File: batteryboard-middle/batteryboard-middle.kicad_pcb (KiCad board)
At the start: 2 copper layers, 46.8 x 46.8 mm, 8 parts, among them J1 Conn_02x05_Odd_Even, J2 Conn_01x02, J3 Conn_01x02, J4 Conn_02x05_Odd_Even

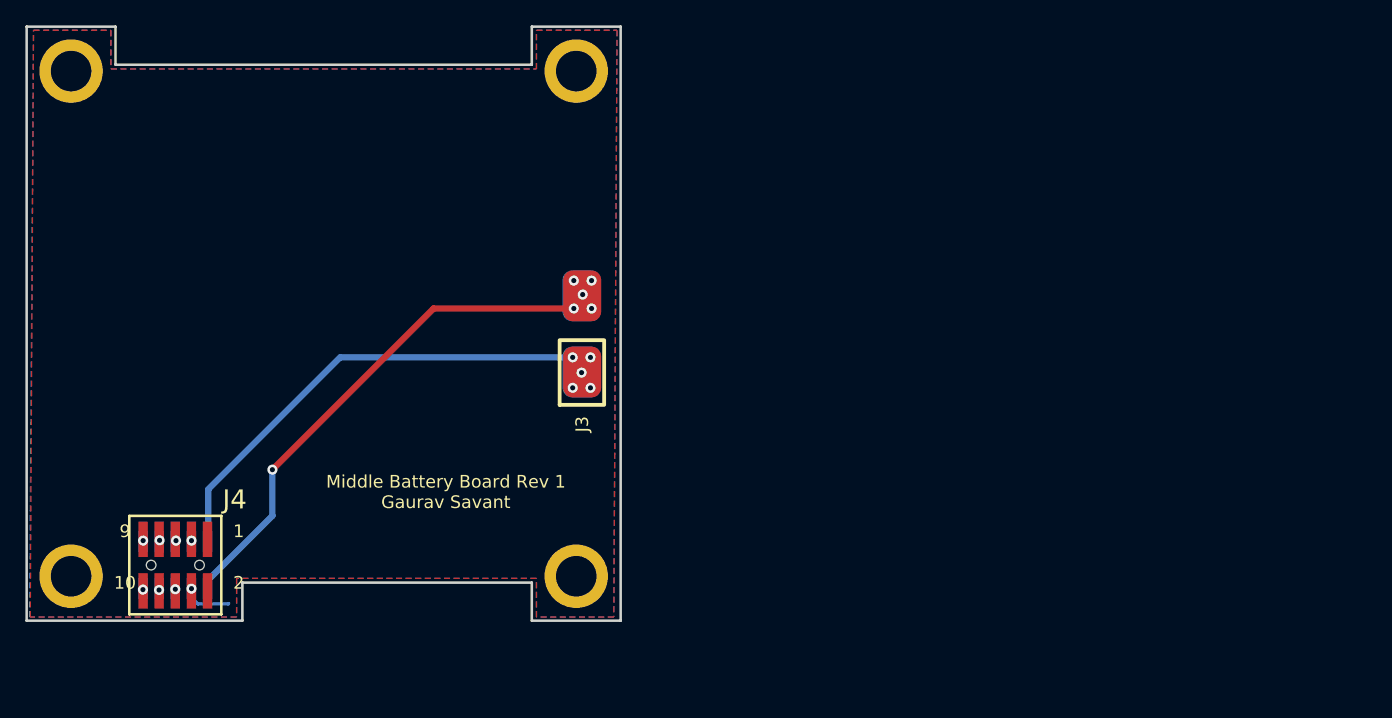
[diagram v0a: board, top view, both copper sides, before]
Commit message: Fixes and cleanup
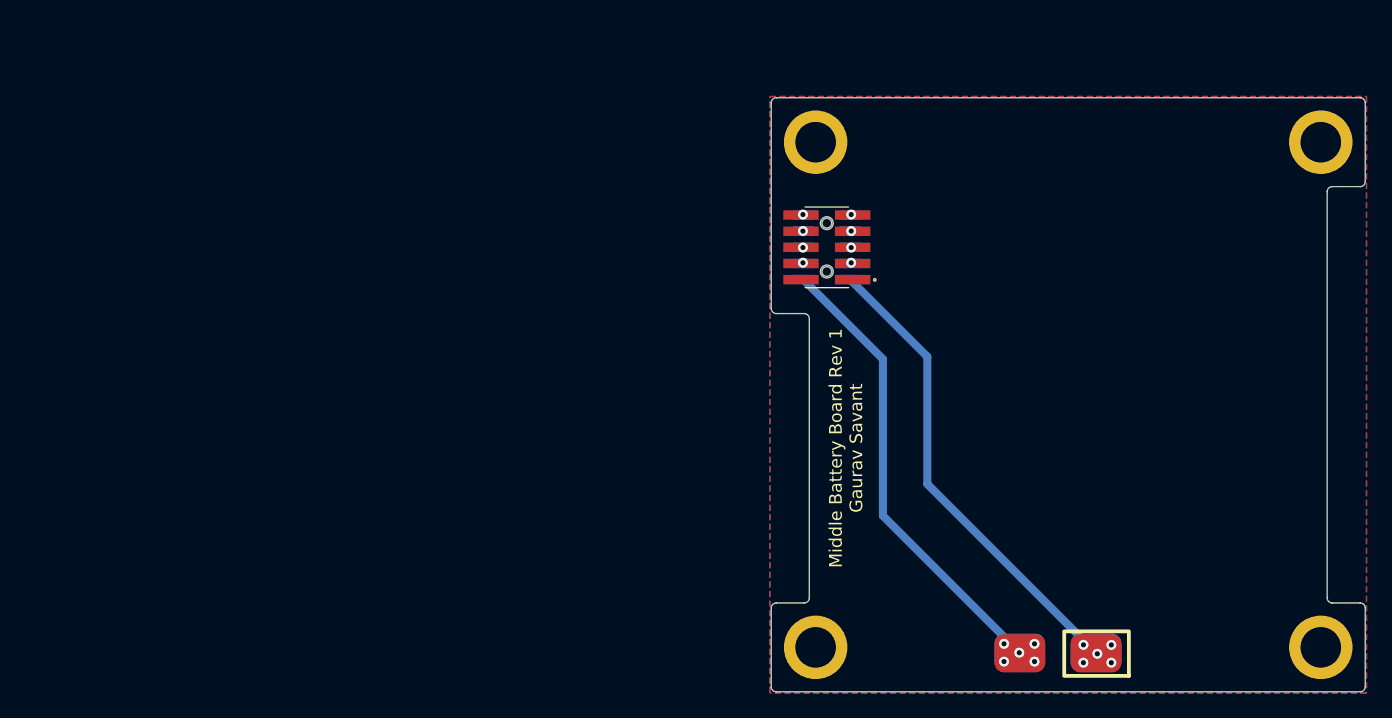
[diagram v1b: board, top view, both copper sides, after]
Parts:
- added Ref**: Val**, custom-footprints:pycubed_mini_half, F.Cu at (147.6, 80.2)
- J4: footprint batteryboard:SAMTEC-FTS-105-01-X-DV -> batteryboard:FTS-105-XX-YY-DV-A
- moved H1 98.6 mm to (166.7, 80.7), turned to -90 degrees
- moved H2 74.2 mm to (166.7, 120.5), turned to -90 degrees
- moved H4 67.9 mm to (126.9, 80.7), turned to -90 degrees
- moved J1 57.1 mm to (127.8, 89.0), turned to 90 degrees
- moved J4 57.1 mm to (127.8, 89.0), turned to 90 degrees
- moved J2 45.2 mm to (146.0, 120.9), turned to 180 degrees
- moved J3 45.1 mm to (146.0, 121.0), turned to 180 degrees
- moved H3 19.7 mm to (126.9, 120.5), turned to -90 degrees
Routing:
- net GND: track 4.49 -> 0.00 mm
- net BATT_N_SW: track 39.9 -> 36.5 mm, vias 6 -> 5
- net BATT_P_SW: track 36.5 -> 37.4 mm
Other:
- outline, holes or cut-outs redrawn
- board text added: "09-JUN-22"
- board text added: "v01"
